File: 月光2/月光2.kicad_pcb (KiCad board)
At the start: 2 copper layers, 40 x 60.5 mm, 73 parts, among them J1 Conn_01x12, J2 Conn_01x12, J3 Conn_01x05, J4 Conn_01x03, J6 Conn_01x02, Q1 Q_Photo_NPN, Q2 Q_Photo_NPN, Q3 Q_Photo_NPN, Q4 Q_Photo_NPN, Q5 IRLML6344TRPBFTR, SW1 SW_Push_Dual_x2, U1 DRV8835, U2 STM32F413CH6, U4 LP5907_DBV, U5 ICM20648, Y1 Crystal_GND23

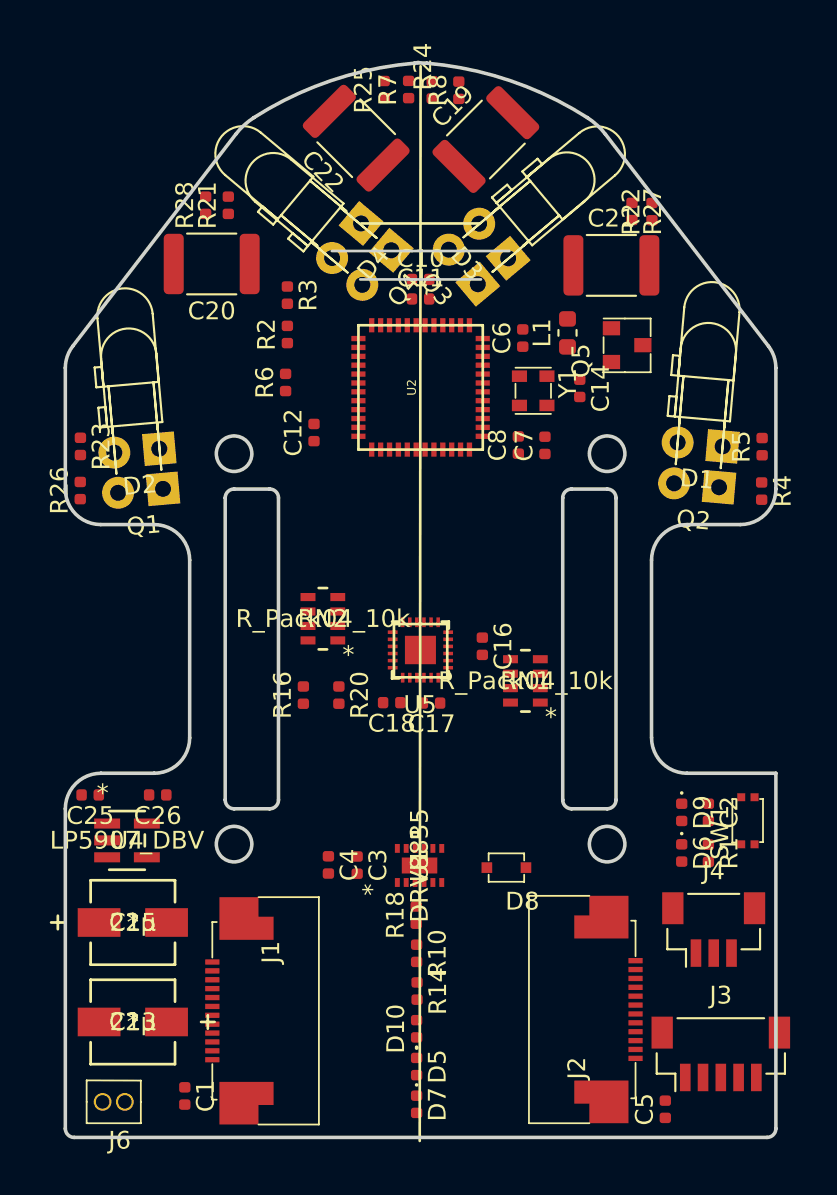
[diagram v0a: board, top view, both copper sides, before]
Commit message: haisenmae
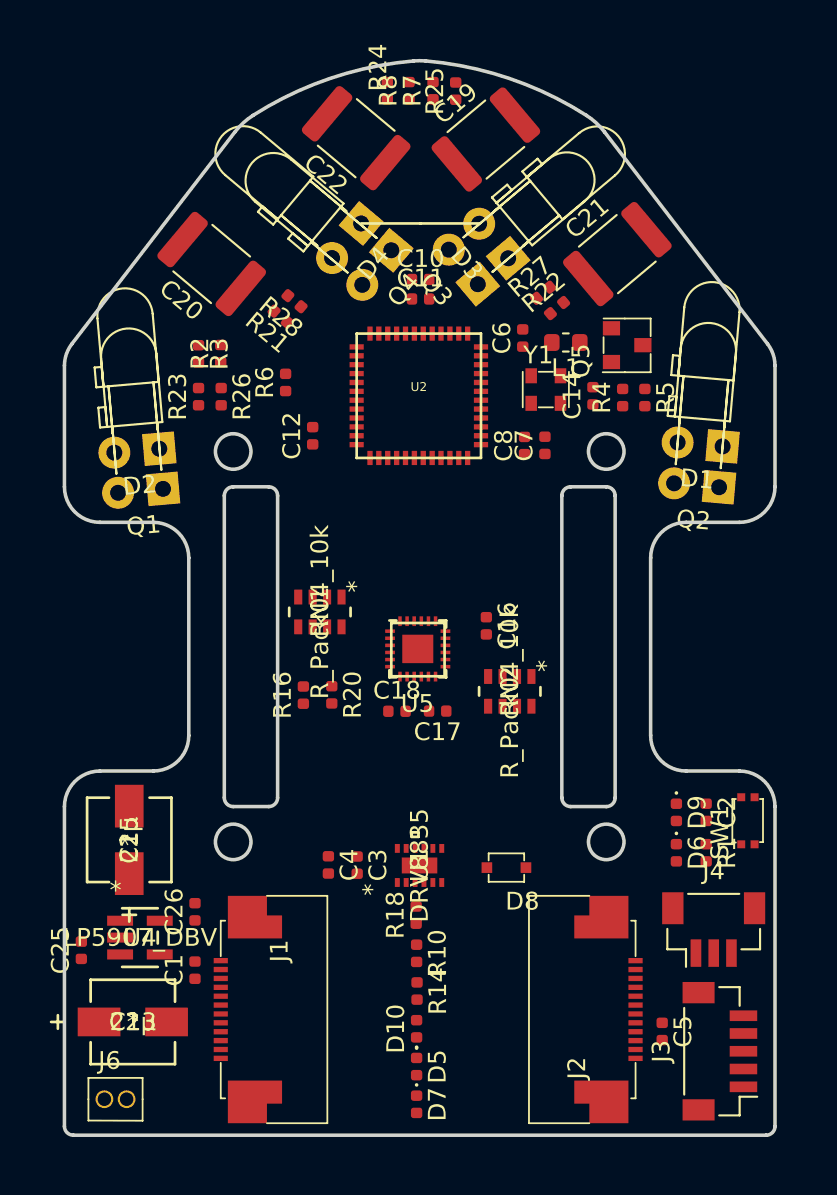
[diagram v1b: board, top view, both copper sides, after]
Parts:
- moved RN1 12.2 mm to (144.3, 118.3), turned to 270 degrees
- moved RN2 11.3 mm to (155.0, 122.8), turned to 270 degrees
- moved R26 9.53 mm to (138.8, 106.2), turned to 270 degrees
- moved R4 9.43 mm to (161.4, 106.2), turned to 90 degrees
- moved C25 8.76 mm to (130.9, 137.4), turned to 90 degrees
- moved R22 7.62 mm to (157.7, 101.2), turned to 40 degrees
- moved R28 7.36 mm to (142.9, 100.8), turned to 140 degrees
- moved R23 7.22 mm to (137.5, 106.2), turned to 90 degrees
- moved R5 7.16 mm to (162.6, 106.2), turned to 270 degrees
- moved C1 7.10 mm to (137.3, 138.5), turned to 90 degrees
- moved R21 6.93 mm to (142.1, 101.7), turned to 140 degrees
- moved C26 6.91 mm to (137.3, 135.2), turned to 90 degrees
- moved R27 6.78 mm to (156.9, 100.3), turned to 40 degrees
- moved R3 5.99 mm to (137.5, 103.8)
- moved U4 5.52 mm to (134.2, 136.7)
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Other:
- outline, holes or cut-outs redrawn
